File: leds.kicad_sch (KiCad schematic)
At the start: 13 parts, among them J13 LED-Ring, J14 LED-Ring, J19 LED-Ring, J21 LED-Ring, J22 LED-Ring, J4 JST XH 3, J8 LED-Ring, U2 74AHCT1G32SE-7

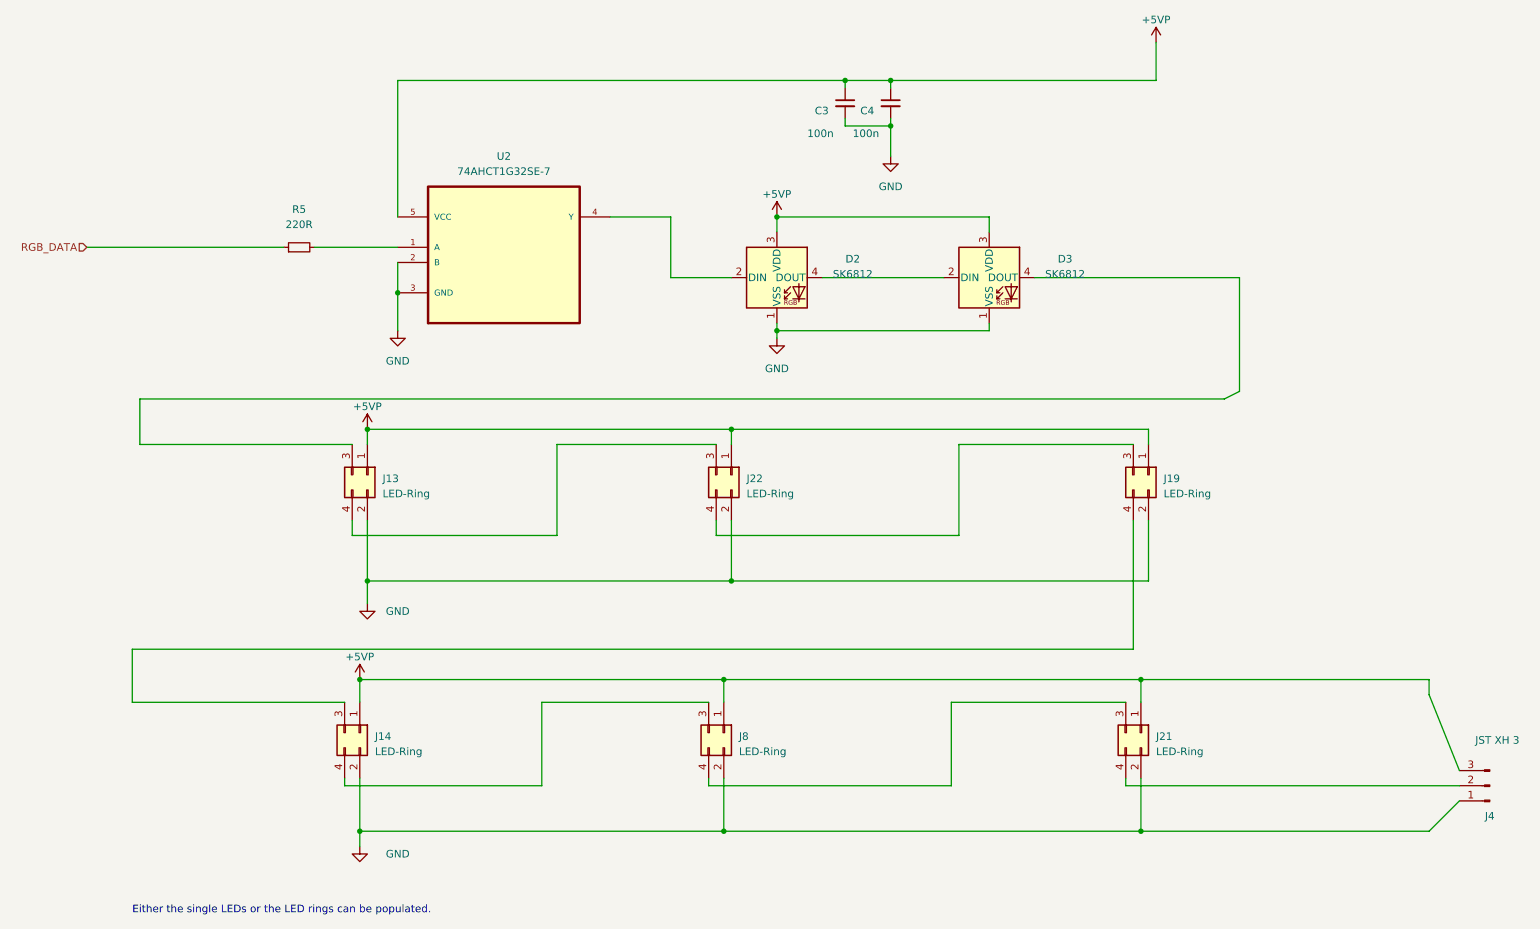
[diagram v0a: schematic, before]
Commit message: Add one Led ring
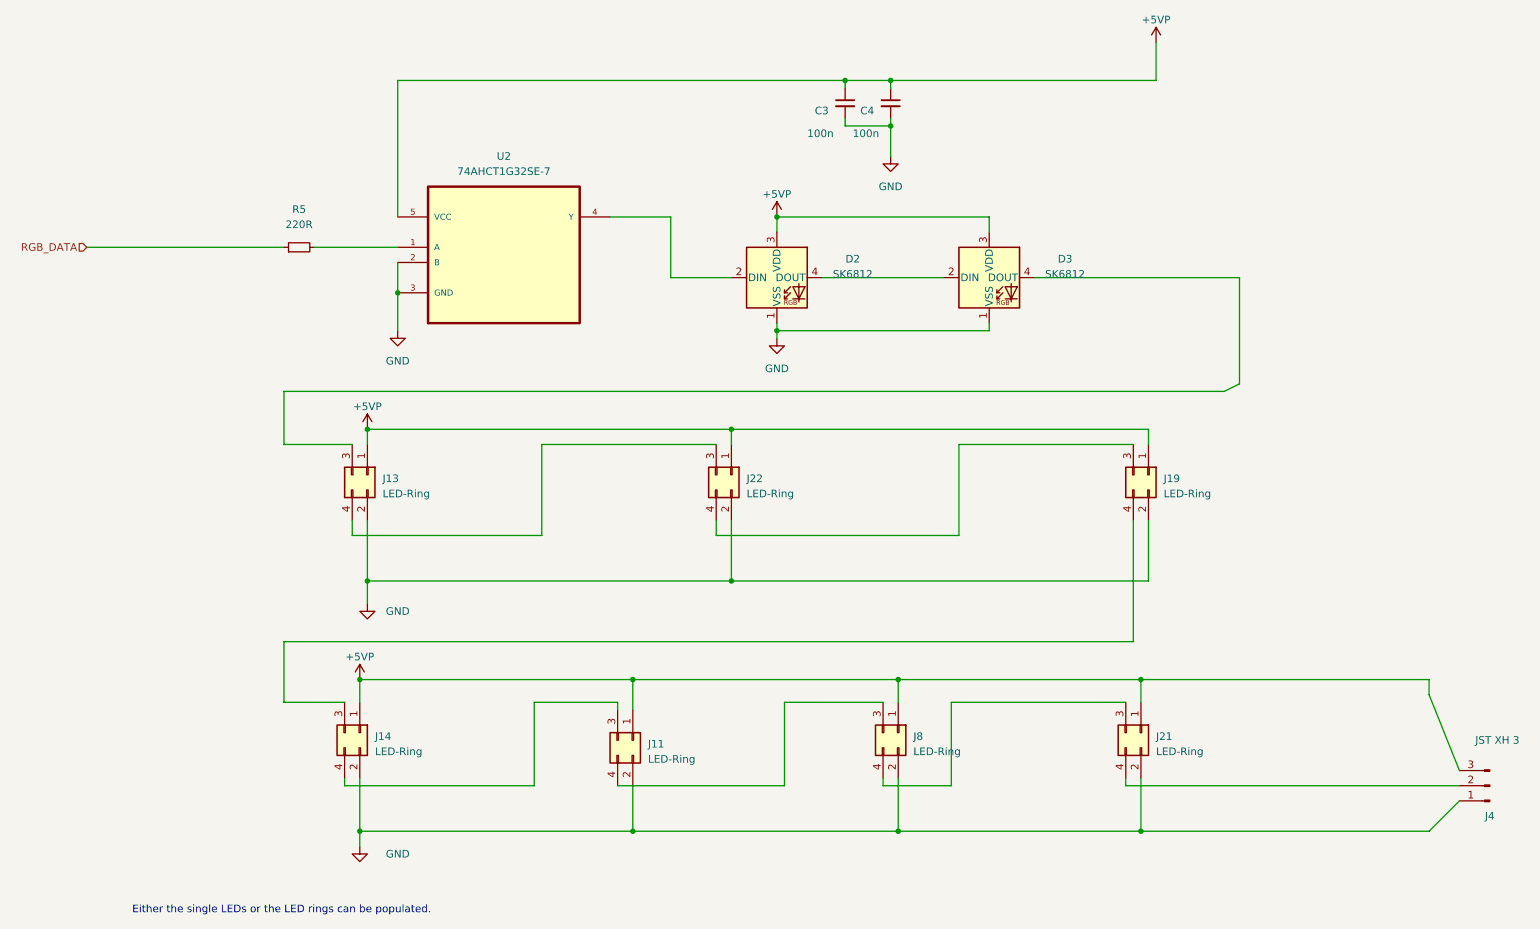
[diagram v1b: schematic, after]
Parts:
- added J11: LED-Ring, Pedalboard Library:Led-Ring, symbol Connector_Generic:Conn_02x02_Odd_Even
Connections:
- net +5VP: now also J11.1 (Pin_1)
- net GND: now also J11.2 (Pin_2)
- net at J14.4 (Pin_4): now also J11.3 (Pin_3); no longer J8.3 (Pin_3)
- new net: J11.4 (Pin_4), J8.3 (Pin_3)
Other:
- moved on the sheet: J8
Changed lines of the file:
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@@
     (comment 2 "License: CERN Open Hardware Licence Version 2 - Permissive")
   )
+  (junction (at 121.92 151.13) (diameter 0) (color 0 0 0 0)
+  )
   (junction (at 138.43 83.82) (diameter 0) (color 0 0 0 0)
   )
@@
   (junction (at 146.05 48.26) (diameter 0) (color 0 0 0 0)
   )
-  (junction (at 137.16 151.13) (diameter 0) (color 0 0 0 0)
-  )
   (junction (at 77.47 83.82) (diameter 0) (color 0 0 0 0)
   )
   (junction (at 138.43 109.22) (diameter 0) (color 0 0 0 0)
   )
+  (junction (at 121.92 125.73) (diameter 0) (color 0 0 0 0)
+  )
   (junction (at 146.05 67.31) (diameter 0) (color 0 0 0 0)
   )
+  (junction (at 166.37 125.73) (diameter 0) (color 0 0 0 0)
+  )
   (junction (at 77.47 109.22) (diameter 0) (color 0 0 0 0)
   )
   (junction (at 76.2 125.73) (diameter 0) (color 0 0 0 0)
   )
-  (junction (at 137.16 125.73) (diameter 0) (color 0 0 0 0)
+  (junction (at 166.37 151.13) (diameter 0) (color 0 0 0 0)
   )
   (junction (at 82.55 60.96) (diameter 0) (color 0 0 0 0)
@@
   (junction (at 165.1 33.02) (diameter 0) (color 0 0 0 0)
   )
-  (wire (pts (xy 137.16 151.13) (xy 207.01 151.13))
-    (stroke (width 0) (type default))
-  )
   (wire (pts (xy 77.47 99.06) (xy 77.47 109.22))
     (stroke (width 0) (type default))
@@
     (stroke (width 0) (type default))
   )
+  (wire (pts (xy 119.38 129.54) (xy 119.38 130.81))
+    (stroke (width 0) (type default))
+  )
   (wire (pts (xy 138.43 99.06) (xy 138.43 109.22))
     (stroke (width 0) (type default))
@@
     (stroke (width 0) (type default))
   )
-  (wire (pts (xy 38.1 129.54) (xy 73.66 129.54))
-    (stroke (width 0) (type default))
-  )
-  (wire (pts (xy 205.74 99.06) (xy 205.74 120.65))
+  (wire (pts (xy 119.38 143.51) (xy 147.32 143.51))
+    (stroke (width 0) (type default))
+  )
+  (wire (pts (xy 205.74 99.06) (xy 205.74 119.38))
     (stroke (width 0) (type default))
   )
@@
     (stroke (width 0) (type default))
   )
-  (wire (pts (xy 134.62 143.51) (xy 175.26 143.51))
+  (wire (pts (xy 163.83 143.51) (xy 175.26 143.51))
     (stroke (width 0) (type default))
   )
@@
     (stroke (width 0) (type default))
   )
+  (wire (pts (xy 63.5 129.54) (xy 73.66 129.54))
+    (stroke (width 0) (type default))
+  )
   (wire (pts (xy 77.47 109.22) (xy 138.43 109.22))
     (stroke (width 0) (type default))
@@
     (stroke (width 0) (type default))
   )
-  (wire (pts (xy 137.16 125.73) (xy 207.01 125.73))
+  (wire (pts (xy 121.92 151.13) (xy 166.37 151.13))
     (stroke (width 0) (type default))
   )
@@
     (stroke (width 0) (type default))
   )
+  (wire (pts (xy 166.37 125.73) (xy 207.01 125.73))
+    (stroke (width 0) (type default))
+  )
   (wire (pts (xy 146.05 48.26) (xy 146.05 50.8))
     (stroke (width 0) (type default))
@@
     (stroke (width 0) (type default))
   )
-  (wire (pts (xy 74.93 101.6) (xy 109.22 101.6))
+  (wire (pts (xy 147.32 129.54) (xy 163.83 129.54))
+    (stroke (width 0) (type default))
+  )
+  (wire (pts (xy 74.93 101.6) (xy 106.68 101.6))
     (stroke (width 0) (type default))
   )
@@
     (stroke (width 0) (type default))
   )
-  (wire (pts (xy 137.16 142.24) (xy 137.16 151.13))
+  (wire (pts (xy 166.37 142.24) (xy 166.37 151.13))
     (stroke (width 0) (type default))
   )
@@
     (stroke (width 0) (type default))
   )
-  (wire (pts (xy 106.68 129.54) (xy 106.68 143.51))
+  (wire (pts (xy 105.41 129.54) (xy 105.41 143.51))
     (stroke (width 0) (type default))
   )
@@
     (stroke (width 0) (type default))
   )
-  (wire (pts (xy 134.62 129.54) (xy 106.68 129.54))
-    (stroke (width 0) (type default))
-  )
-  (wire (pts (xy 223.52 77.47) (xy 220.98 78.74))
+  (wire (pts (xy 223.52 76.2) (xy 220.98 77.47))
     (stroke (width 0) (type default))
   )
@@
     (stroke (width 0) (type default))
   )
-  (wire (pts (xy 137.16 125.73) (xy 137.16 129.54))
+  (wire (pts (xy 166.37 125.73) (xy 166.37 129.54))
     (stroke (width 0) (type default))
   )
@@
     (stroke (width 0) (type default))
   )
+  (wire (pts (xy 121.92 125.73) (xy 121.92 130.81))
+    (stroke (width 0) (type default))
+  )
+  (wire (pts (xy 63.5 119.38) (xy 63.5 129.54))
+    (stroke (width 0) (type default))
+  )
   (wire (pts (xy 73.66 142.24) (xy 73.66 143.51))
     (stroke (width 0) (type default))
@@
     (stroke (width 0) (type default))
   )
-  (wire (pts (xy 39.37 78.74) (xy 220.98 78.74))
+  (wire (pts (xy 63.5 77.47) (xy 220.98 77.47))
     (stroke (width 0) (type default))
   )
@@
     (stroke (width 0) (type default))
   )
-  (wire (pts (xy 39.37 86.36) (xy 74.93 86.36))
+  (wire (pts (xy 63.5 86.36) (xy 74.93 86.36))
     (stroke (width 0) (type default))
   )
@@
     (stroke (width 0) (type default))
   )
+  (wire (pts (xy 166.37 151.13) (xy 207.01 151.13))
+    (stroke (width 0) (type default))
+  )
+  (wire (pts (xy 121.92 143.51) (xy 121.92 151.13))
+    (stroke (width 0) (type default))
+  )
   (wire (pts (xy 157.48 33.02) (xy 165.1 33.02))
     (stroke (width 0) (type default))
@@
     (stroke (width 0) (type default))
   )
-  (wire (pts (xy 38.1 120.65) (xy 38.1 129.54))
-    (stroke (width 0) (type default))
-  )
   (wire (pts (xy 207.01 142.24) (xy 207.01 151.13))
     (stroke (width 0) (type default))
@@
     (stroke (width 0) (type default))
   )
+  (wire (pts (xy 105.41 129.54) (xy 119.38 129.54))
+    (stroke (width 0) (type default))
+  )
   (wire (pts (xy 207.01 125.73) (xy 255.27 125.73))
     (stroke (width 0) (type default))
@@
     (stroke (width 0) (type default))
   )
-  (wire (pts (xy 134.62 142.24) (xy 134.62 143.51))
+  (wire (pts (xy 163.83 142.24) (xy 163.83 143.51))
     (stroke (width 0) (type default))
   )
@@
     (stroke (width 0) (type default))
   )
+  (wire (pts (xy 121.92 125.73) (xy 166.37 125.73))
+    (stroke (width 0) (type default))
+  )
   (wire (pts (xy 157.48 31.75) (xy 157.48 33.02))
     (stroke (width 0) (type default))
   )
-  (wire (pts (xy 73.66 143.51) (xy 106.68 143.51))
+  (wire (pts (xy 73.66 143.51) (xy 105.41 143.51))
     (stroke (width 0) (type default))
   )
@@
     (stroke (width 0) (type default))
   )
-  (wire (pts (xy 38.1 120.65) (xy 205.74 120.65))
+  (wire (pts (xy 63.5 119.38) (xy 205.74 119.38))
     (stroke (width 0) (type default))
   )
@@
     (stroke (width 0) (type default))
   )
-  (wire (pts (xy 76.2 125.73) (xy 137.16 125.73))
+  (wire (pts (xy 76.2 125.73) (xy 121.92 125.73))
     (stroke (width 0) (type default))
   )
@@
     (stroke (width 0) (type default))
   )
-  (wire (pts (xy 39.37 78.74) (xy 39.37 86.36))
-    (stroke (width 0) (type default))
-  )
-  (wire (pts (xy 135.89 86.36) (xy 109.22 86.36))
+  (wire (pts (xy 63.5 77.47) (xy 63.5 86.36))
+    (stroke (width 0) (type default))
+  )
+  (wire (pts (xy 135.89 86.36) (xy 106.68 86.36))
     (stroke (width 0) (type default))
   )
@@
     (stroke (width 0) (type default))
   )
-  (wire (pts (xy 223.52 58.42) (xy 223.52 77.47))
+  (wire (pts (xy 223.52 58.42) (xy 223.52 76.2))
+    (stroke (width 0) (type default))
+  )
+  (wire (pts (xy 147.32 143.51) (xy 147.32 129.54))
     (stroke (width 0) (type default))
   )
@@
     (stroke (width 0) (type default))
   )
-  (wire (pts (xy 76.2 151.13) (xy 137.16 151.13))
-    (stroke (width 0) (type default))
-  )
-  (wire (pts (xy 109.22 86.36) (xy 109.22 101.6))
+  (wire (pts (xy 76.2 151.13) (xy 121.92 151.13))
+    (stroke (width 0) (type default))
+  )
+  (wire (pts (xy 106.68 86.36) (xy 106.68 101.6))
     (stroke (width 0) (type default))
   )
@@
     )
   )
-  (symbol (lib_id "Connector_Generic:Conn_02x02_Odd_Even") (at 137.16 134.62 270) (unit 1)
-    (in_bom yes) (on_board yes) (dnp no) (fields_autoplaced)
-    (property "Reference" "J8" (at 139.7 135.255 90)
-      (effects (font (size 1.27 1.27)) (justify left))
-    )
-    (property "Value" "LED-Ring" (at 139.7 137.795 90)
-      (effects (font (size 1.27 1.27)) (justify left))
-    )
-    (property "Footprint" "Pedalboard Library:Led-Ring" (at 137.16 134.62 0)
-      (effects (font (size 1.27 1.27)) hide)
-    )
-    (property "Datasheet" "~" (at 137.16 134.62 0)
+  (symbol (lib_id "Connector_Generic:Conn_02x02_Odd_Even") (at 166.37 134.62 270) (unit 1)
+    (in_bom yes) (on_board yes) (dnp no) (fields_autoplaced)
+    (property "Reference" "J8" (at 168.91 135.255 90)
+      (effects (font (size 1.27 1.27)) (justify left))
+    )
+    (property "Value" "LED-Ring" (at 168.91 137.795 90)
+      (effects (font (size 1.27 1.27)) (justify left))
+    )
+    (property "Footprint" "Pedalboard Library:Led-Ring" (at 166.37 134.62 0)
+      (effects (font (size 1.27 1.27)) hide)
+    )
+    (property "Datasheet" "~" (at 166.37 134.62 0)
       (effects (font (size 1.27 1.27)) hide)
     )
@@
         )
       )
+    )
+  )
+  (symbol (lib_id "Connector_Generic:Conn_02x02_Odd_Even") (at 121.92 135.89 270) (unit 1)
+    (in_bom yes) (on_board yes) (dnp no) (fields_autoplaced)
+    (property "Reference" "J11" (at 124.46 136.525 90)
+      (effects (font (size 1.27 1.27)) (justify left))
+    )
+    (property "Value" "LED-Ring" (at 124.46 139.065 90)
+      (effects (font (size 1.27 1.27)) (justify left))
+    )
+    (property "Footprint" "Pedalboard Library:Led-Ring" (at 121.92 135.89 0)
+      (effects (font (size 1.27 1.27)) hide)
+    )
+    (property "Datasheet" "~" (at 121.92 135.89 0)
+      (effects (font (size 1.27 1.27)) hide)
+    )
+    (pin "1")
+    (pin "2")
+    (pin "3")
+    (pin "4")
+    (instances
+      (project "pedalboard-hw"
+        (path "/df521c2a-9827-4355-b809-366f4b88d5d7/539b926e-3ef4-477a-b921-49e2b2b26dfc"
+          (reference "J11") (unit 1)
+        )
+      )
